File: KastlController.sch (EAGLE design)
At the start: 17 parts

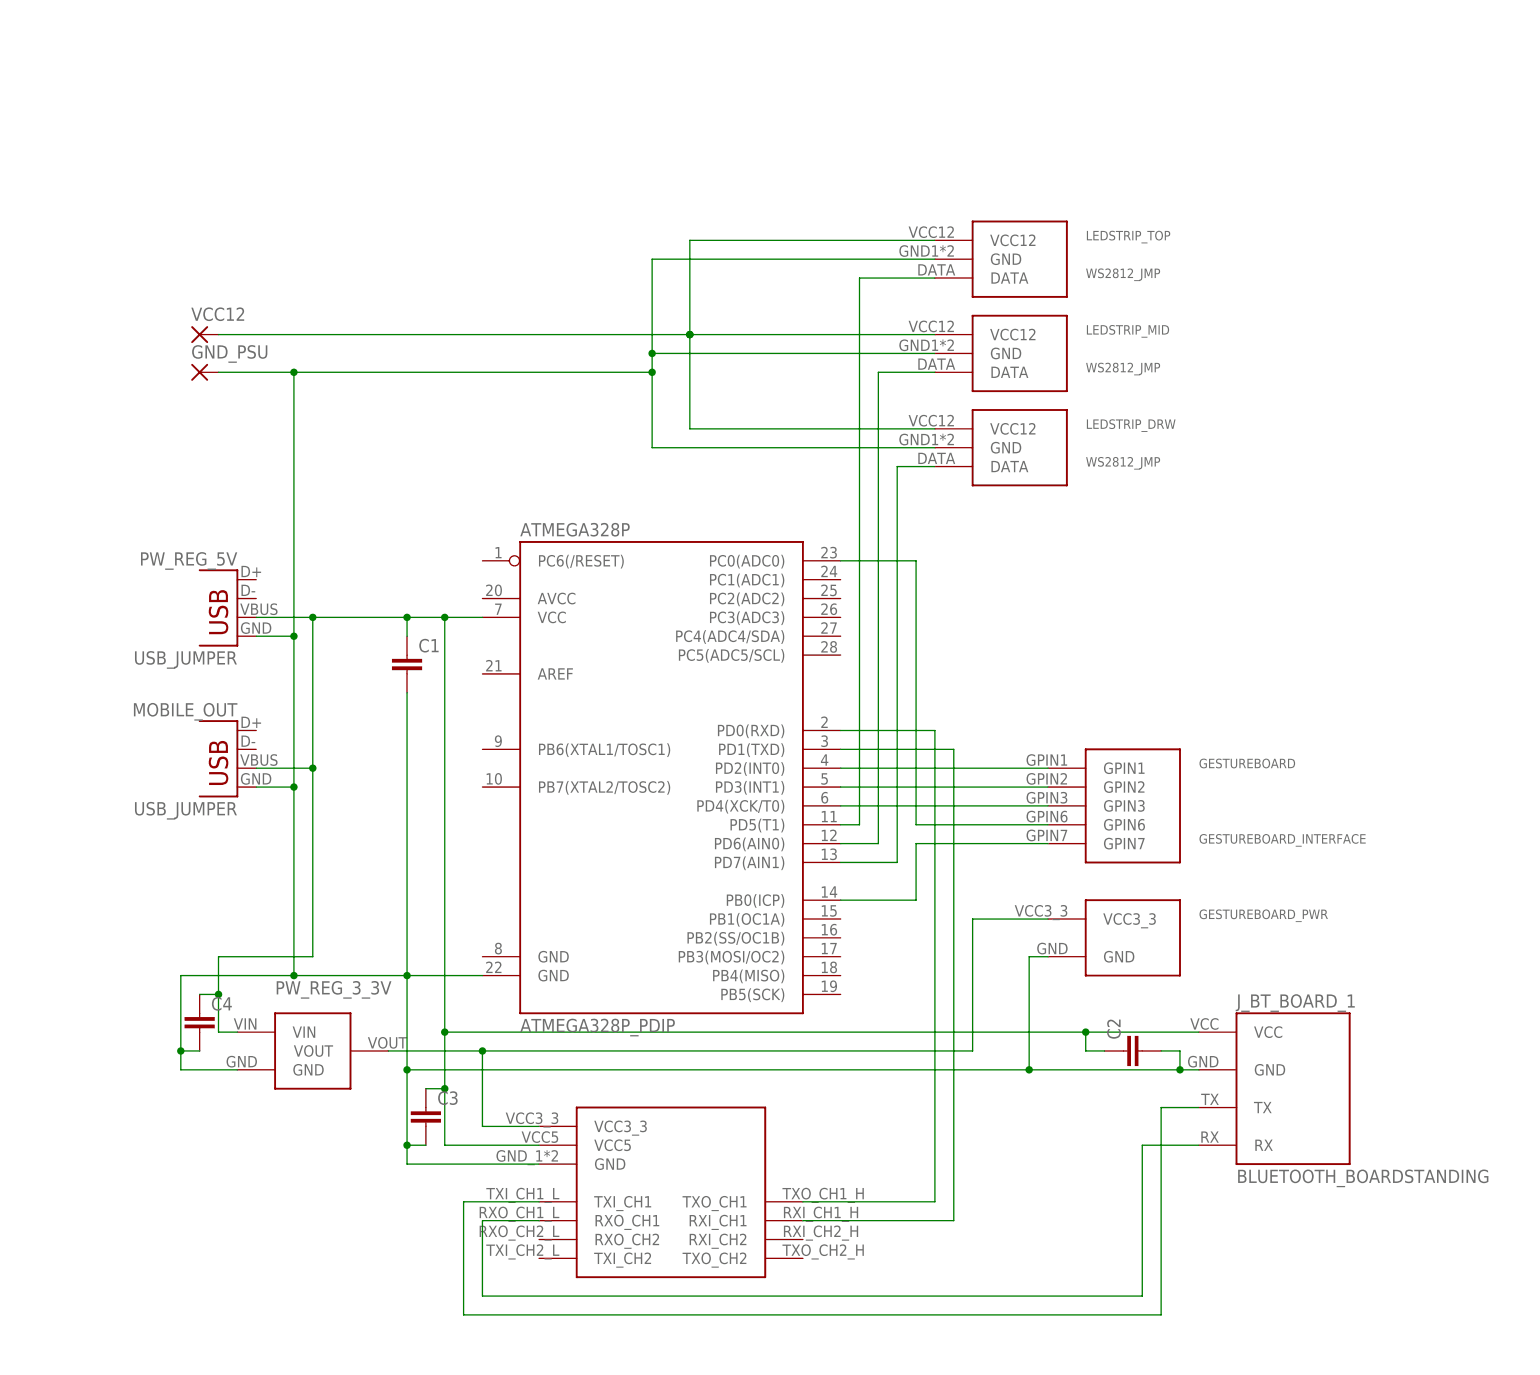
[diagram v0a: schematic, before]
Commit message: Update KastlController.sch
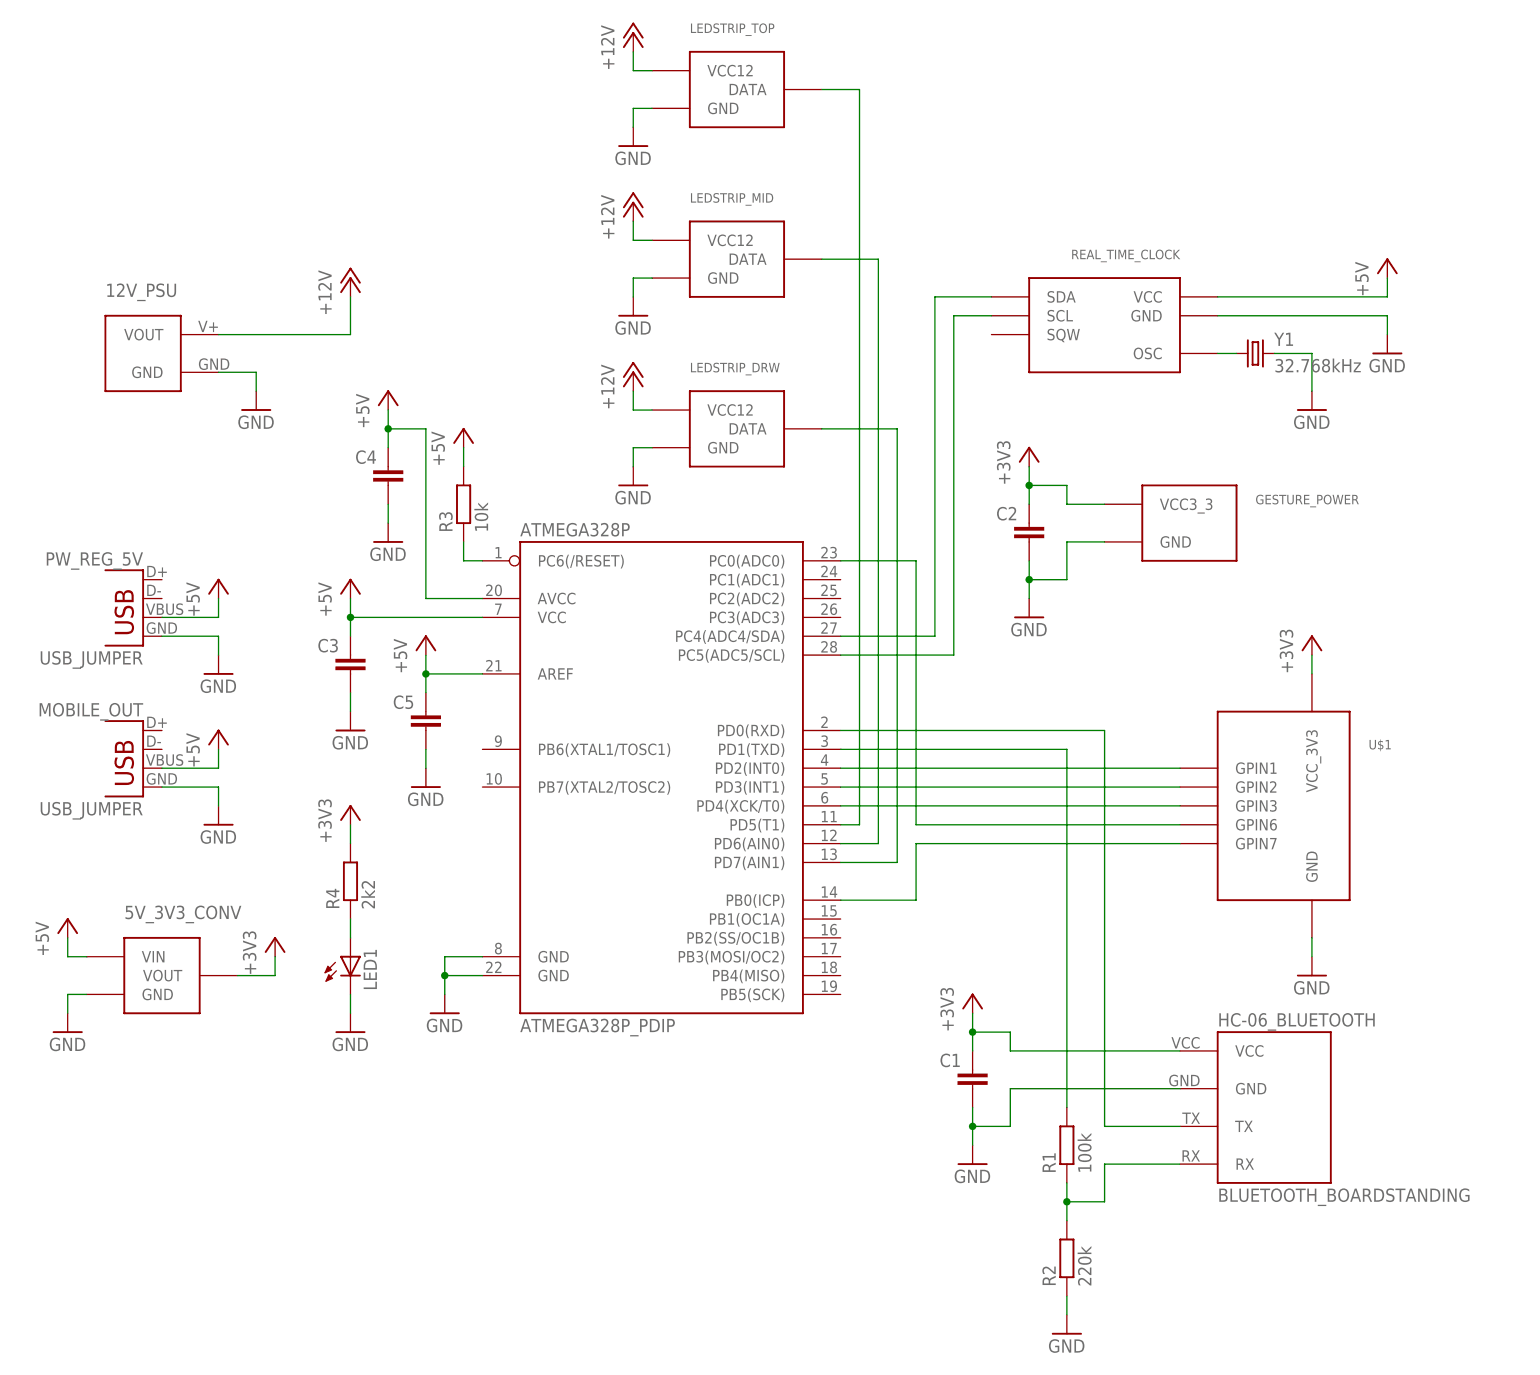
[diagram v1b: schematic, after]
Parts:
- removed GESTUREBOARD: GESTUREBOARD_INTERFACE, gestureBoardInterface_Kastl:GESTUREBOARD_INTERFACE
- removed GESTUREBOARD_PWR: GESTUREBOARD_POWER, gestureBoardInterface_Kastl:GESTUREBOARD_POWER
- removed GND_PSU, VCC12: (no value), wirepad:2,54/1,0
- removed J_BT_BOARD_1: BLUETOOTH_BOARDSTANDING, Bluetooth_HC-06:BLUETOOTH_BOARDSTANDING
- removed PW_REG_3_3V: STEPDOWN_5V-3_3V, 5V3_3V_stepdown:STEPDOWN_5V-3_3V
- added 12V_PSU: PWR_CONNECTOR, PowerConnector:PWR_CONNECTOR
- added 5V_3V3_CONV: STEPDOWN_5V-3_3V, 5V3_3V_stepdown:STEPDOWN_5V-3_3V
- added C5: (no value), htl3r-discrete:C-EU_025-024X044
- added GESTURE_POWER: GESTUREBOARD_POWER, gestureBoardInterface_Kastl:GESTUREBOARD_POWER
- added HC-06_BLUETOOTH: BLUETOOTH_BOARDSTANDING, Bluetooth_HC-06:BLUETOOTH_BOARDSTANDING
- added LED1: (no value), htl3r-discrete:LEDS_5MM
- added R1: 100k, htl3r-discrete:R-EU_0204/2V
- added R2: 220k, htl3r-discrete:R-EU_0204/2V
- added R3: 10k, htl3r-discrete:R-EU_0204/2V
- added R4: 2k2, htl3r-discrete:R-EU_0204/2V
- added REAL_TIME_CLOCK: DS3231_RTC_MODULE, DS3231_RTC:DS3231_RTC_MODULE
- added Y1: 32.768kHz, SparkFun-FreqCtrl:CRYSTAL3.2X1.5MM
- U$1: value 3_3/5V_LEVELCONVERTER -> GESTUREBOARD; device LogicLevelConv_Kastl:3_3/5V_LEVELCONVERTER -> gestureBoardInterface_Kastl:GESTUREBOARD
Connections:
- removed net VCC12: LEDSTRIP_DRW.VCC12, LEDSTRIP_MID.VCC12, LEDSTRIP_TOP.VCC12, VCC12.P
- removed net VCC5: ATMEGA328P.VCC, C1.1, C2.1, C3.1, C4.1, J_BT_BOARD_1.VCC, MOBILE_OUT.VBUS, PW_REG_3_3V.VIN, PW_REG_5V.VBUS, U$1.VCC5
- new net +12V: 12V_PSU.VOUT, LEDSTRIP_DRW.VCC12, LEDSTRIP_MID.VCC12, LEDSTRIP_TOP.VCC12
- new net +3V3: 5V_3V3_CONV.VOUT, C1.1, C2.1, GESTURE_POWER.VCC3_3, HC-06_BLUETOOTH.VCC, U$1.VCC_3V3
- new net +5V: 5V_3V3_CONV.VIN, ATMEGA328P.AREF, ATMEGA328P.AVCC, ATMEGA328P.VCC, C3.1, C4.1, C5.1, MOBILE_OUT.VBUS, PW_REG_5V.VBUS, R3.2, REAL_TIME_CLOCK.VCC
- new net N$13: ATMEGA328P.PC4(ADC4/SDA), REAL_TIME_CLOCK.SDA
- new net N$15: ATMEGA328P.PC5(ADC5/SCL), REAL_TIME_CLOCK.SCL
- new net N$16: HC-06_BLUETOOTH.RX, R1.1, R2.2
- net GND: now also 12V_PSU.GND, 5V_3V3_CONV.GND, ATMEGA328P.GND@1, C5.2, GESTURE_POWER.GND, HC-06_BLUETOOTH.GND, LED1.C, R2.1, REAL_TIME_CLOCK.GND, Y1.2; no longer GESTUREBOARD_PWR.GND, GND_PSU.P, J_BT_BOARD_1.GND, PW_REG_3_3V.GND
- net N$10: now also LED1.A, R4.1; no longer ATMEGA328P.PD1(TXD), U$1.RXI_CH1
- net N$11: now also REAL_TIME_CLOCK.OSC, Y1.1; no longer J_BT_BOARD_1.TX, U$1.TXI_CH1
- net N$12: now also ATMEGA328P.PC6(/RESET), R3.1; no longer J_BT_BOARD_1.RX, U$1.RXO_CH1
- net N$14: now also ATMEGA328P.PD0(RXD), HC-06_BLUETOOTH.TX; no longer GESTUREBOARD_PWR.VCC3_3, PW_REG_3_3V.VOUT, U$1.VCC3_3
- net N$3: now also U$1.GPIN1; no longer GESTUREBOARD.GPIN1
- net N$4: now also U$1.GPIN2; no longer GESTUREBOARD.GPIN2
- net N$5: now also U$1.GPIN3; no longer GESTUREBOARD.GPIN3
- net N$6: now also U$1.GPIN6; no longer GESTUREBOARD.GPIN6
- net N$7: now also U$1.GPIN7; no longer GESTUREBOARD.GPIN7
- net N$9: now also ATMEGA328P.PD1(TXD), R1.2; no longer ATMEGA328P.PD0(RXD), U$1.TXO_CH1
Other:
- moved on the sheet: C1, C2, C3, C4, MOBILE_OUT, PW_REG_5V
